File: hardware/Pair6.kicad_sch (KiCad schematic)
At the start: 10 parts, among them IC6 TPS2HCS08AQPWPRQ1, J17 Conn_01x02, J9 Conn_01x02

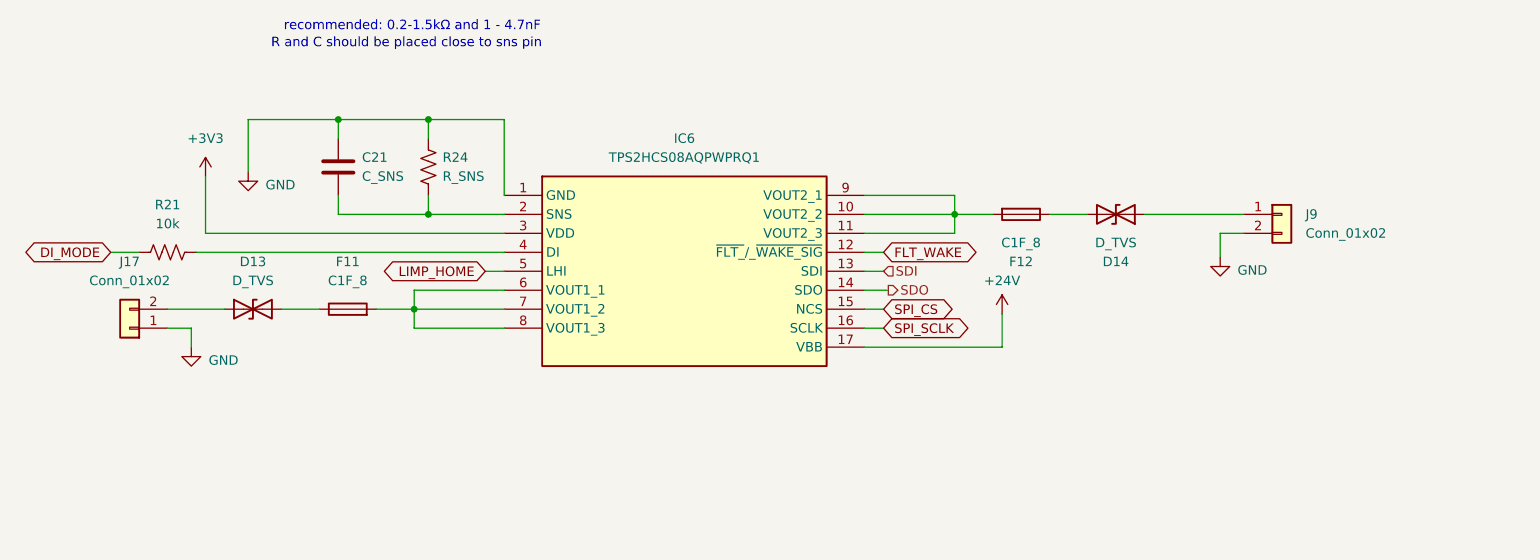
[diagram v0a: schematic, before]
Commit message: aesthetic added
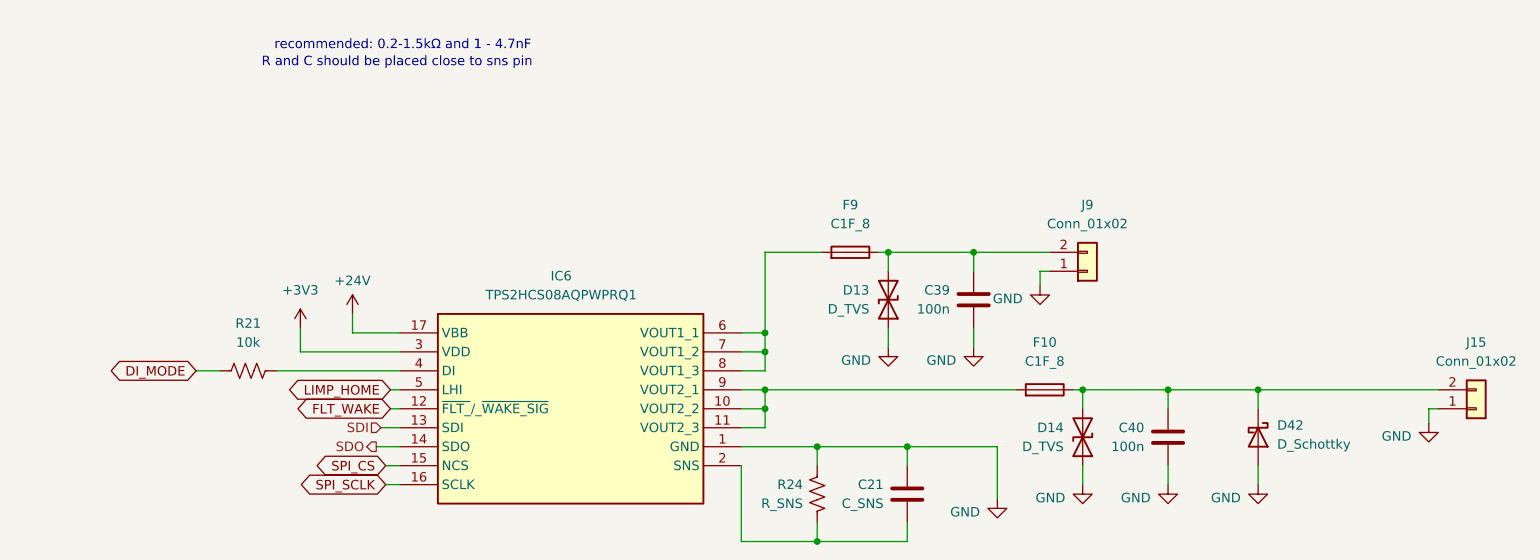
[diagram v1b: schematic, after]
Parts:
- removed F11, F12: C1F_8, Fuse:Fuse_1206_3216Metric, symbol PowerDistributionUnitLib:C1F_8
- removed J17: Conn_01x02, symbol Connector_Generic:Conn_01x02
- added C39, C40: 100n, symbol Device:C
- added D42: D_Schottky, symbol Device:D_Schottky
- added F10, F9: C1F_8, Fuse:Fuse_1206_3216Metric, symbol PowerDistributionUnitLib:C1F_8
- added J15: Conn_01x02, symbol Connector_Generic:Conn_01x02
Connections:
- net GND: now also D13.1 (A1), D14.1 (A1), J9.1 (Pin_1), C39.1, C40.1, D42.2 (A), J15.1 (Pin_1); no longer J9.2 (Pin_2)
- net at D14.2 (A2): now also C40.2, D42.1 (K), F10.1, J15.2 (Pin_2)
- net at IC6.10 (VOUT2_2), IC6.11 (VOUT2_3), IC6.9 (VOUT2_1): now also F10.2
- net at IC6.6 (VOUT1_1), IC6.7 (VOUT1_2), IC6.8 (VOUT1_3): now also F9.2
- net at D13.2 (A2): now also J9.2 (Pin_2), C39.2, F9.1
